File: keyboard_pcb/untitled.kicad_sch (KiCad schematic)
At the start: 33 parts, among them J1 USB_C_Receptacle_USB2.0_16P, J2 Conn_01x02, SW1 Reset, U1 NCP1117-3.3_SOT223, U2 RP2040, U3 W25Q128JVS, Y1 Crystal_GND24

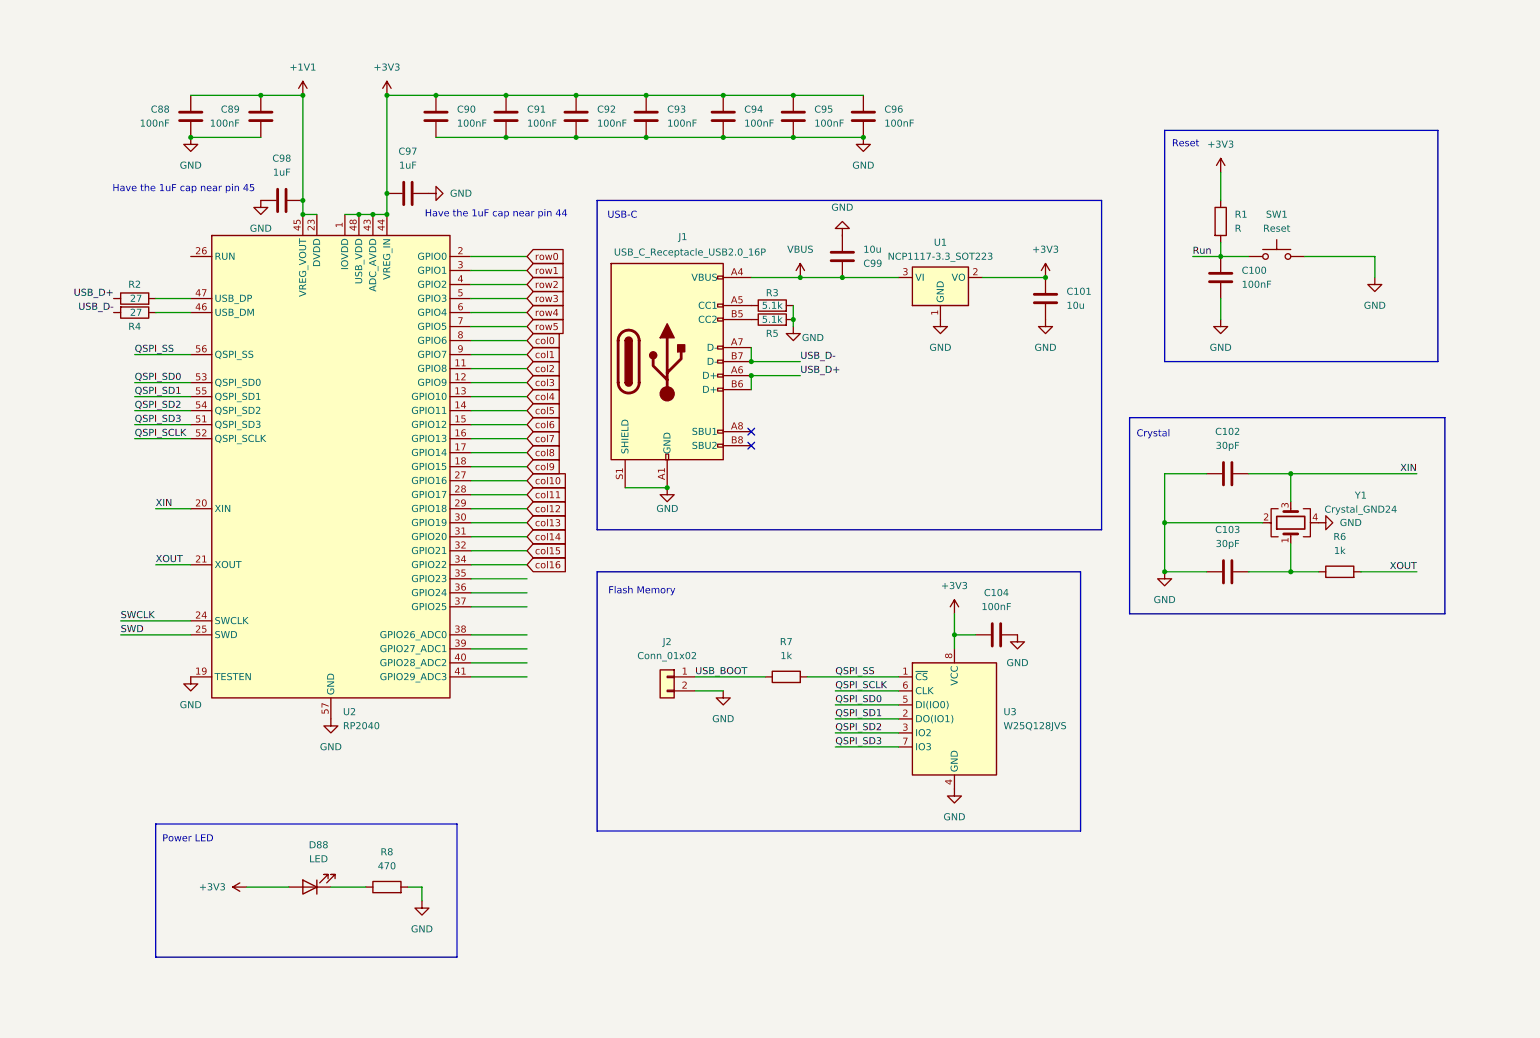
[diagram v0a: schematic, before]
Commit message: updated schematic
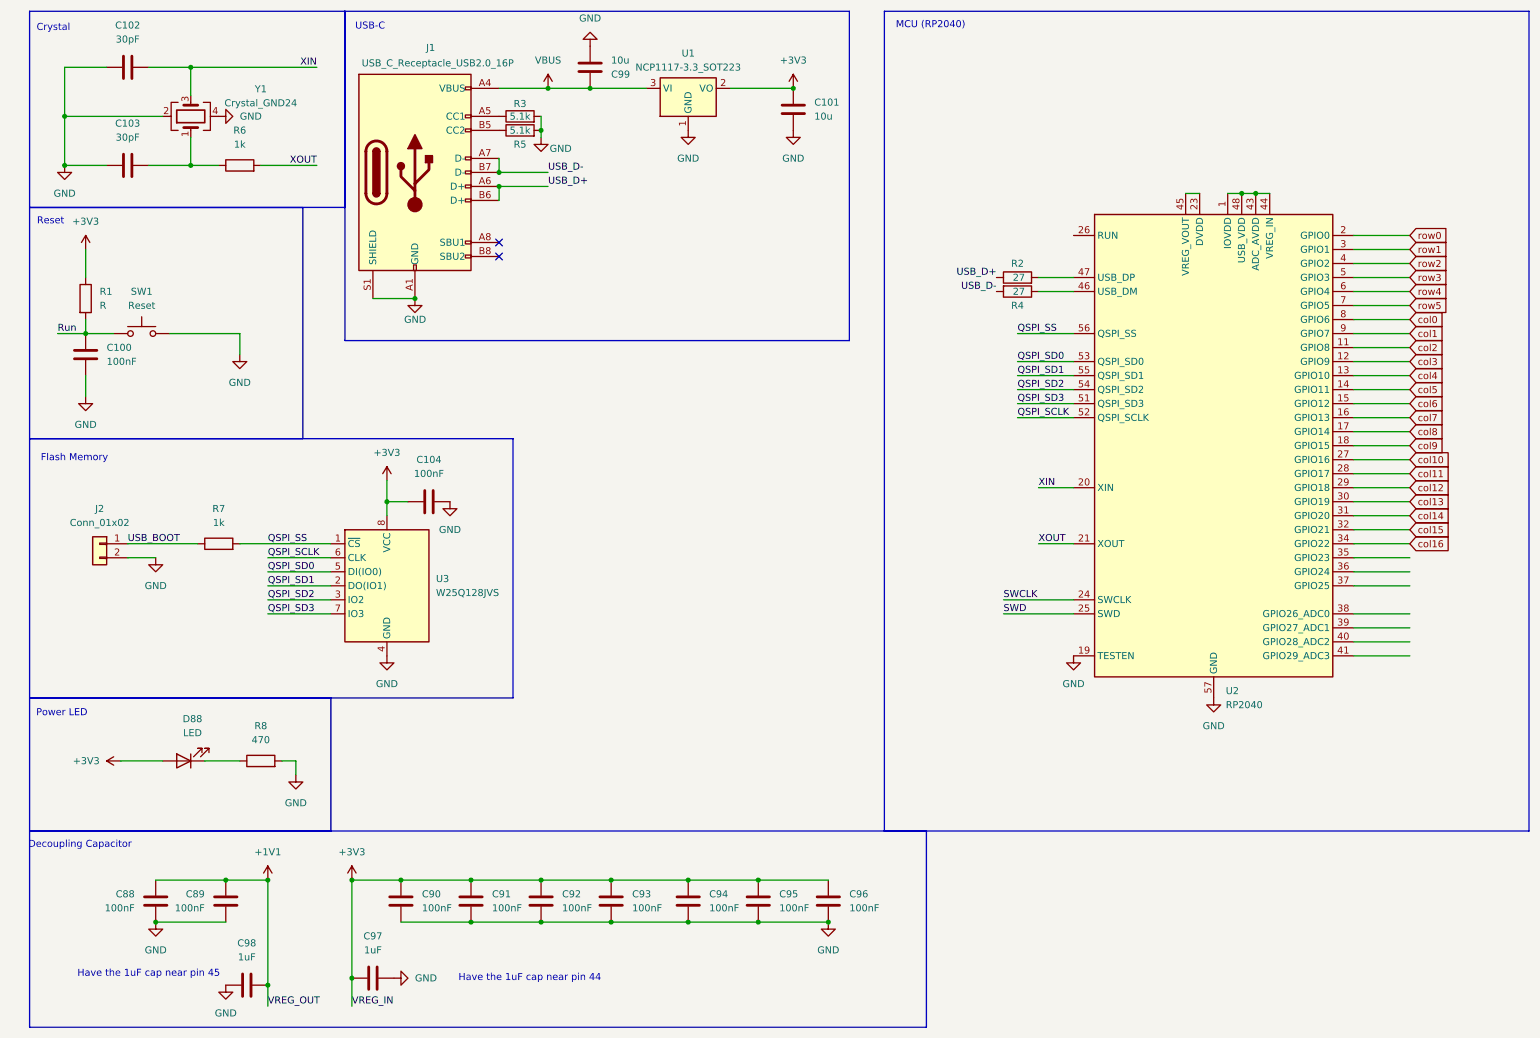
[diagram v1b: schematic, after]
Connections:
- net +1V1: no longer U2.23 (DVDD), U2.45 (VREG_VOUT), U2.50 (DVDD)
- net +3V3: no longer U2.1 (IOVDD), U2.10 (IOVDD), U2.22 (IOVDD), U2.33 (IOVDD), U2.42 (IOVDD), U2.43 (ADC_AVDD), U2.44 (VREG_IN), U2.48 (USB_VDD), U2.49 (IOVDD)
- new net: U2.1 (IOVDD), U2.10 (IOVDD), U2.22 (IOVDD), U2.33 (IOVDD), U2.42 (IOVDD), U2.43 (ADC_AVDD), U2.44 (VREG_IN), U2.48 (USB_VDD), U2.49 (IOVDD)
- new net: U2.23 (DVDD), U2.45 (VREG_VOUT), U2.50 (DVDD)
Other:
- note added: "Decoupling Capacitor"
- note added: "MCU (RP2040)"
- moved on the sheet: C100, C101, C102, C103, C104, C88, C89, C90, C91, C92, C93, C94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
